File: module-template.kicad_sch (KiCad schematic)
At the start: 0 parts

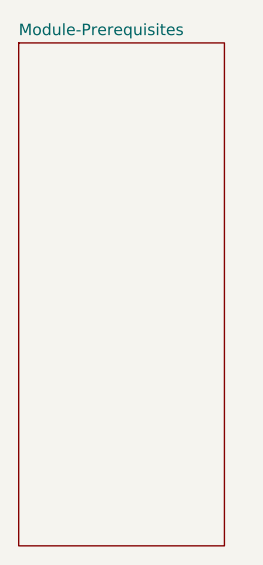
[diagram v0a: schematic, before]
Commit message: Work on Prerequisites sheet
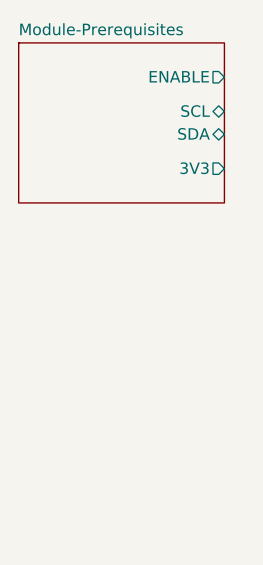
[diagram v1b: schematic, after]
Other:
- sheet Module-Prerequisites ports: added 3V3, ENABLE, SCL, SDA; removed none
- title: Module Template -> Module Prerequisites
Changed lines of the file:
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@@
 (kicad_sch (version 20230121) (generator eeschema)
-  (paper "USLetter")
+  (paper "A5")
   (title_block
-    (title "Module Template")
-    (date "~")
+    (title "Module Prerequisites")
+    (date "2023-08-16")
     (company "Fieldkit")
     (comment 1 "Bradley Gawthrop")
     (comment 2 "module-template")
   )
-  (sheet (at 15.24 17.78) (size 22.86 55.88) (fields_autoplaced)
+  (sheet (at 15.24 17.78) (size 22.86 17.78) (fields_autoplaced)
     (stroke (width 0.1524) (type solid))
     (fill (color 0 0 0 0.0000))
@@
       (effects (font (size 1.27 1.27)) (justify left bottom))
     )
-    (property "Sheetfile" "module-prerequisites.kicad_sch" (at 15.24 74.2446 0)
+    (property "Sheetfile" "module-prerequisites.kicad_sch" (at 15.24 36.1446 0)
       (effects (font (size 1.27 1.27)) (justify left top) hide)
     )
+    (pin "SDA" bidirectional (at 38.1 27.94 0)
+      (effects (font (size 1.27 1.27)) (justify right))
+    )
+    (pin "SCL" bidirectional (at 38.1 25.4 0)
+      (effects (font (size 1.27 1.27)) (justify right))
+    )
+    (pin "3V3" output (at 38.1 31.75 0)
+      (effects (font (size 1.27 1.27)) (justify right))
+    )
+    (pin "ENABLE" output (at 38.1 21.59 0)
+      (effects (font (size 1.27 1.27)) (justify right))
+    )
     (instances

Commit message: Finished prerequisites. Started component placement.
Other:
- title: Module Prerequisites -> Module Template
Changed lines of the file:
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@@
   (paper "A5")
   (title_block
-    (title "Module Prerequisites")
+    (title "Module Template")
     (date "2023-08-16")
     (company "Fieldkit")

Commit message: Small aesthetic channges, and KiCad version update.
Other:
- company: Fieldkit -> (none)
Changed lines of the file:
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@@
-(kicad_sch (version 20230121) (generator eeschema)
-  (paper "A5")
-  (title_block
-    (title "Module Template")
-    (date "2023-08-16")
-    (company "Fieldkit")
-    (comment 1 "Bradley Gawthrop")
-    (comment 2 "module-template")
-  )
-  (sheet (at 15.24 17.78) (size 22.86 17.78) (fields_autoplaced)
-    (stroke (width 0.1524) (type solid))
-    (fill (color 0 0 0 0.0000))
-    (property "Sheetname" "Module-Prerequisites" (at 15.24 17.0684 0)
-      (effects (font (size 1.27 1.27)) (justify left bottom))
-    )
-    (property "Sheetfile" "module-prerequisites.kicad_sch" (at 15.24 36.1446 0)
-      (effects (font (size 1.27 1.27)) (justify left top) hide)
-    )
-    (pin "SDA" bidirectional (at 38.1 27.94 0)
-      (effects (font (size 1.27 1.27)) (justify right))
-    )
-    (pin "SCL" bidirectional (at 38.1 25.4 0)
-      (effects (font (size 1.27 1.27)) (justify right))
-    )
-    (pin "3V3" output (at 38.1 31.75 0)
-      (effects (font (size 1.27 1.27)) (justify right))
-    )
-    (pin "ENABLE" output (at 38.1 21.59 0)
-      (effects (font (size 1.27 1.27)) (justify right))
-    )
-    (instances
-      (project "module-template"
-        (path "/0fe8f37a-a549-417a-a51a-96b485ec4340" (page "2"))
-      )
-    )
-  )
-  (sheet_instances
-    (path "/" (page "1"))
-  )
+(kicad_sch
+	(version 20231120)
+	(generator "eeschema")
+	(generator_version "8.0")
+	(paper "A5")
+	(title_block
+		(title "Module Template")
+		(date "2023-08-17")
+	)
+	(sheet
+		(at 15.24 17.78)
+		(size 22.86 17.78)
+		(fields_autoplaced yes)
+		(stroke
+			(width 0.1524)
+			(type solid)
+		)
+		(fill
+			(color 0 0 0 0.0000)
+		)
+		(property "Sheetname" "Module-Prerequisites"
+			(at 15.24 17.0684 0)
+			(effects
+				(font
+					(size 1.27 1.27)
+				)
+				(justify left bottom)
+			)
+		)
+		(property "Sheetfile" "module-prerequisites.kicad_sch"
+			(at 15.24 36.1446 0)
+			(effects
+				(font
+					(size 1.27 1.27)
+				)
+				(justify left top)
+				(hide yes)
+			)
+		)
+		(pin "SDA" bidirectional
+			(at 38.1 27.94 0)
+			(effects
+				(font
+					(size 1.27 1.27)
+				)
+				(justify right)
+			)
+		)
+		(pin "SCL" bidirectional
+			(at 38.1 25.4 0)
+			(effects
+				(font
+					(size 1.27 1.27)
+				)
+				(justify right)
+			)
+		)
+		(pin "3V3" output
+			(at 38.1 31.75 0)
+			(effects
+				(font
+					(size 1.27 1.27)
+				)
+				(justify right)
+			)
+		)
+		(pin "ENABLE" output
+			(at 38.1 21.59 0)
+			(effects
+				(font
+					(size 1.27 1.27)
+				)
+				(justify right)
+			)
+		)
+		(instances
+			(project "module-template"
+				(path "/0fe8f37a-a549-417a-a51a-96b485ec4340"
+					(page "2")
+				)
+			)
+		)
+	)
+	(sheet_instances
+		(path "/"
+			(page "1")
+		)
+	)
 )
